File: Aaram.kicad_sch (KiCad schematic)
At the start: 51 parts, among them J1 Conn_01x03, J2 Conn_01x02, J3 AC_OUT, J4 SWITCH_IN, J5 5V_OUT, J6 PSU_AC_IN, J8 SPARE_PINS, K1 10A cube relay, K2 10A cube relay, K3 10A cube relay, Q1 BT136-600, Q2 2N2222A, Q3 2N2222A, Q4 2N2222A, U1 ESP32-DevKitC, U2 TLP281-4GB_F_

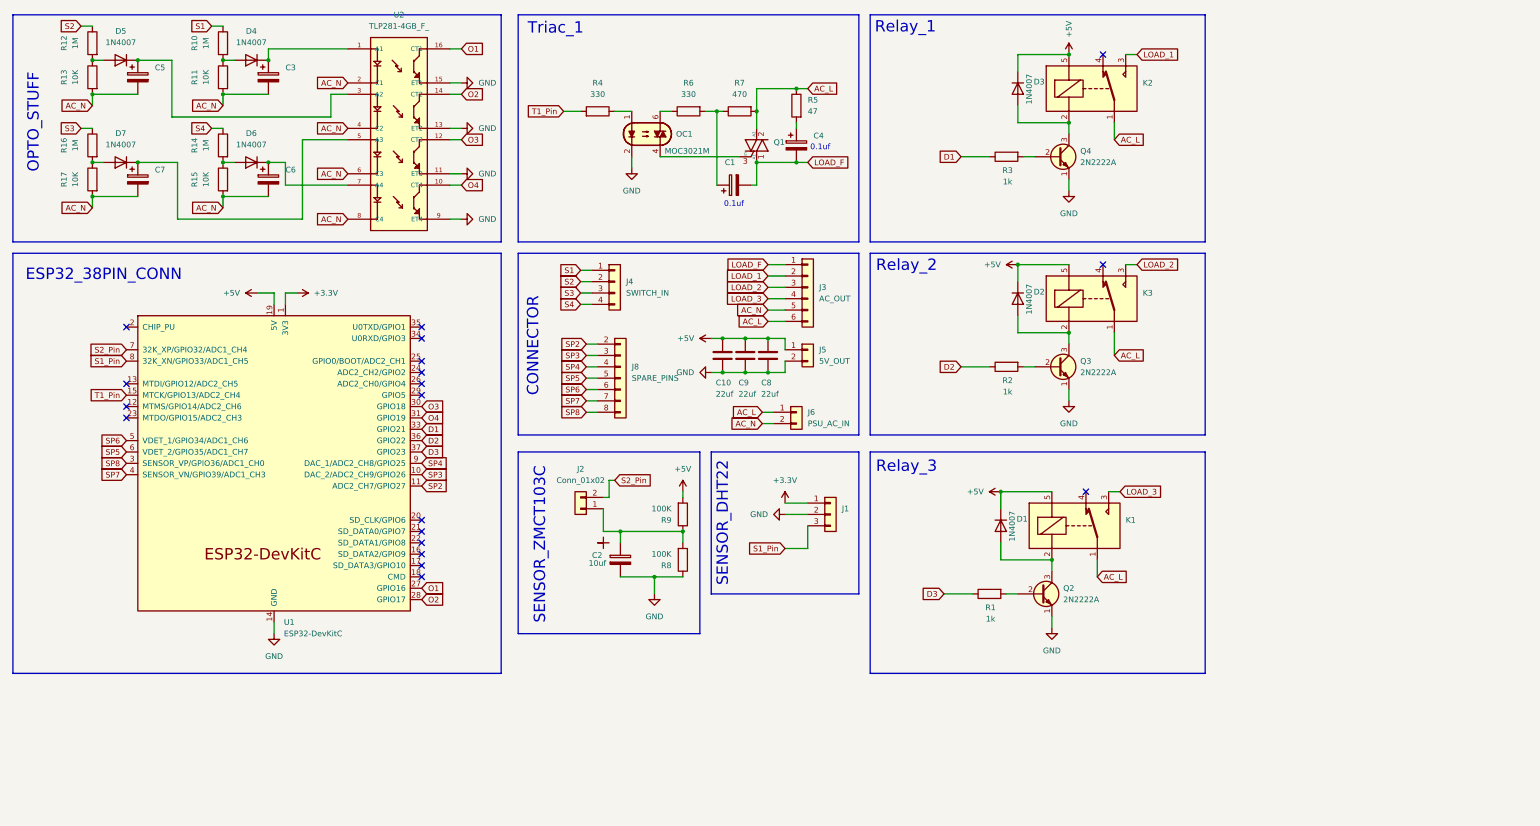
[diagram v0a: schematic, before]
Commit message: Major Update (#2)
* Updated mostly everything

* Big Update

* Major Update

- Removed All 3D related files for now.
- Updated the Schematics and PCB
- Updated the assets

* File move

* Updated readme
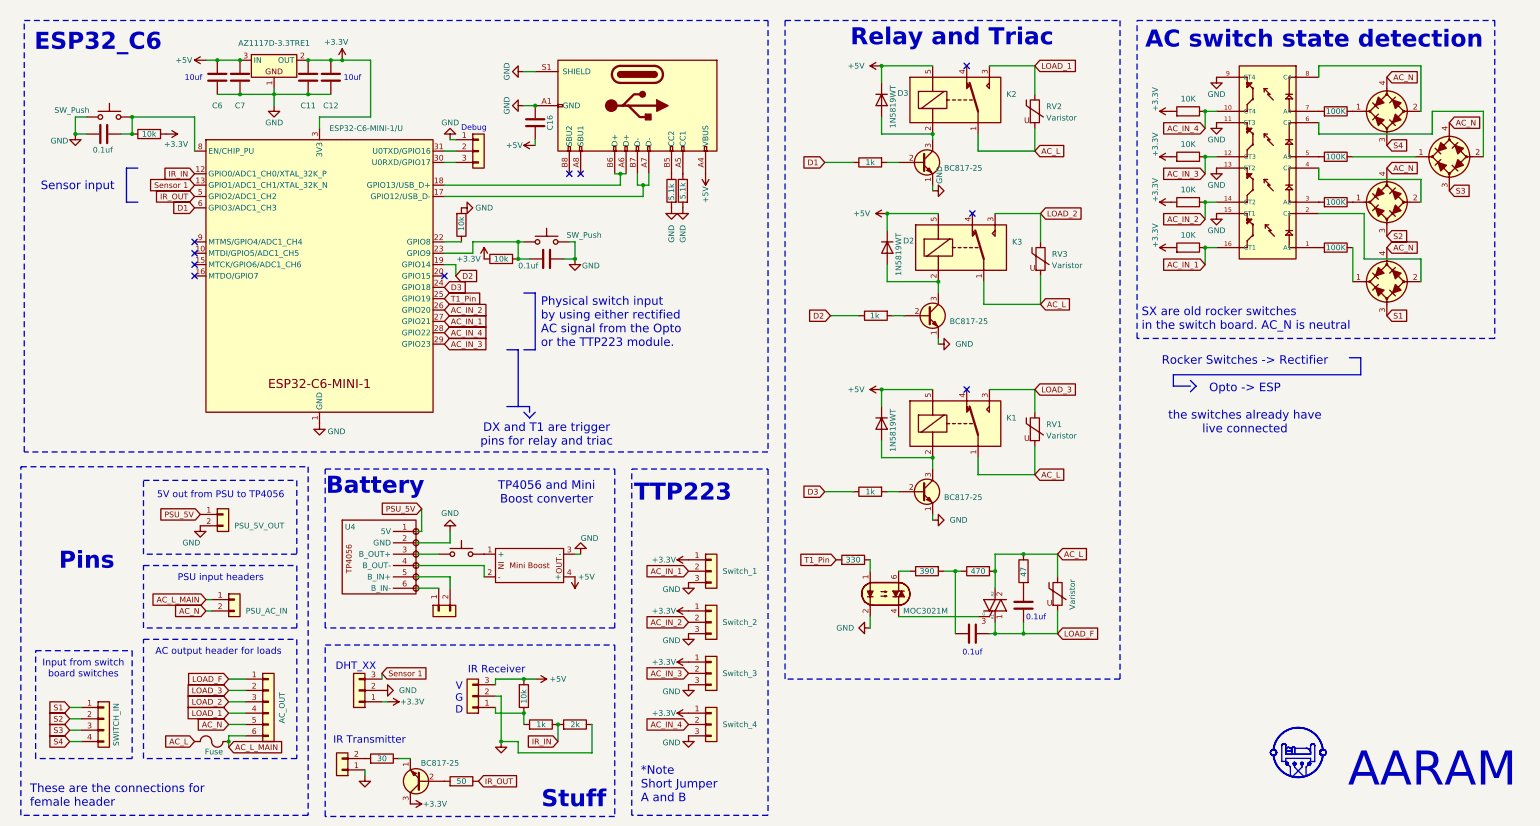
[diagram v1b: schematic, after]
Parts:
- removed C10, C8, C9: 22uf, PCM_Capacitor_SMD_Handsoldering_AKL:C_1206_3216Metric_Pad1.42x1.75mm, symbol PCM_Capacitor_AKL:C_1206
- removed C2: 10uf, Xicor_Custom stuff:Film_Cap_13x13mm_P5.00mm, symbol PCM_Capacitor_AKL:CP_Radial_D10.0mm_P5.00mm
- removed C3, C5, C6, C7: CP_Axial_L10.0mm_D4.5mm_P15.00mm, Xicor_Custom stuff:Axial_Capacitor_P10mm_W4.5mm, symbol PCM_Capacitor_AKL:CP_Axial_L10.0mm_D4.5mm_P15.00mm
- removed D4, D5, D6, D7: 1N4007, Diode_SMD:D_SMA_Handsoldering, symbol Diode:1N4007
- removed J8: SPARE_PINS, Connector_PinHeader_2.54mm:PinHeader_1x08_P2.54mm_Vertical, symbol Connector_Generic:Conn_01x08
- removed U1: ESP32-DevKitC, Xicor_Custom stuff:ESP32_38Pin, symbol PCM_Espressif:ESP32-DevKitC
- removed U2: TLP281-4GB_F_, Xicor_Custom stuff:SOIC127P700X210-16N, symbol TLP281-4GB_F_:TLP281-4GB_F_
- added C11, C12, C6, C7: 10uf, PCM_Capacitor_SMD_Handsoldering_AKL:C_1206_3216Metric_Pad1.42x1.75mm, symbol PCM_Capacitor_AKL:C_Generic
- added C16: 1uf, PCM_Capacitor_SMD_Handsoldering_AKL:C_1206_3216Metric_Pad1.42x1.75mm, symbol PCM_Capacitor_AKL:C_Generic
- added C18, C19: 0.1uf, PCM_Capacitor_SMD_Handsoldering_AKL:C_1206_3216Metric_Pad1.42x1.75mm, symbol PCM_Capacitor_AKL:C_1206
- added D10, D11, D8, D9: MB6S, PCM_Diode_SMD_AKL:Diode_Bridge_MBS, symbol PCM_Diode_Bridge_AKL:MB6S
- added F1: Fuse, Xicor_Custom stuff:BLX-A, symbol PCM_Device_AKL:Fuse
- added J10, J11: Conn_01x03, Connector_PinSocket_2.54mm:PinSocket_1x03_P2.54mm_Vertical, symbol Connector_Generic:Conn_01x03
- added J8: USB_C_Receptacle_USB2.0_16P, Connector_USB:USB_C_Receptacle_GCT_USB4105-xx-A_16P_TopMnt_Horizontal, symbol Connector:USB_C_Receptacle_USB2.0_16P
- added J9: Conn_01x02, Connector_PinSocket_2.54mm:PinSocket_1x02_P2.54mm_Vertical, symbol Connector_Generic:Conn_01x02
- added Q5: BC817-25, Package_TO_SOT_SMD:TSOT-23_HandSoldering, symbol PCM_Transistor_BJT_AKL:2N2222A
- added R19, R23: 100K, PCM_Resistor_SMD_AKL:R_2512_6332Metric_Pad1.52x3.35mm_HandSolder, symbol PCM_Resistor_AKL:R_1206
- added R20, R25, R26, R27: 10K, PCM_Resistor_SMD_AKL:R_1206_3216Metric_Pad1.42x1.75mm_HandSolder, symbol PCM_Resistor_AKL:R_1206
- added R21, R22: 10k, PCM_Resistor_SMD_AKL:R_1206_3216Metric_Pad1.42x1.75mm_HandSolder, symbol PCM_Resistor_AKL:R_1206
- added RV1, RV2, RV3, RV4: Varistor, Xicor_Custom stuff:Varistor_10D431K, symbol Device:Varistor
- added SW1, SW4: SW_Push, Xicor_Custom stuff:Tactile switch 6x3, symbol Switch:SW_Push
- added SW2: SW_Push, Xicor_Custom stuff:SMD Tactile switch, symbol Switch:SW_Push
- added Switch_1, Switch_2, Switch_3, Switch_4: Conn_01x03_Socket, Connector_JST:JST_SH_BM03B-SRSS-TB_1x03-1MP_P1.00mm_Vertical, symbol Connector_Generic:Conn_01x03
- added U1: ESP32-C6-MINI-1/U, PCM_Espressif:ESP32-C6-MINI-1, symbol PCM_Espressif:ESP32-C6-MINI-1/U
- added U2: AZ1117D-3.3TRE1, PCM_Package_TO_SOT_SMD_AKL:TO-252-2, symbol PCM_Voltage_Regulator_AKL:AZ1117D-3.3TRE1
- added U3: ~, Xicor_Custom stuff:Mini_Boost, symbol Xicor_Custom:Mini_Boost
- added U4: ~, Xicor_Custom stuff:TP4056-18650, symbol Xicor_Custom:TP4056-18650
- added U5: TLP281-4GB_F_, Xicor_Custom stuff:SOP127P780X200-16N, symbol TLP281-4GB_F_:TLP281-4GB_F_
- C1: symbol PCM_Capacitor_AKL:CP_Axial_L10.0mm_D4.5mm_P15.00mm -> PCM_Capacitor_AKL:C_3640
- C4: symbol PCM_Capacitor_AKL:CP_Axial_L10.0mm_D4.5mm_P15.00mm -> PCM_Capacitor_US_AKL:C_0805
- D1, D2, D3: value 1N4007 -> 1N5819WT
- J5: value 5V_OUT -> PSU_5V_OUT
- Q2, Q3, Q4: value 2N2222A -> BC817-25; footprint PCM_Package_TO_SOT_SMD_AKL:SOT-23_BigPads -> Package_TO_SOT_SMD:TSOT-23_HandSoldering
- R1, R2, R3, R4: footprint PCM_Capacitor_SMD_Handsoldering_AKL:C_1206_3216Metric_Pad1.42x1.75mm -> PCM_Resistor_SMD_AKL:R_1206_3216Metric_Pad1.42x1.75mm_HandSolder
- R10, R16: value 1M -> 10k; footprint PCM_Capacitor_SMD_Handsoldering_AKL:C_1206_3216Metric_Pad1.42x1.75mm -> PCM_Resistor_SMD_AKL:R_1206_3216Metric_Pad1.42x1.75mm_HandSolder
- R11: value 10K -> 30; footprint PCM_Capacitor_SMD_Handsoldering_AKL:C_1206_3216Metric_Pad1.42x1.75mm -> PCM_Resistor_SMD_AKL:R_1206_3216Metric_Pad1.42x1.75mm_HandSolder
- R12, R14: value 1M -> 5.1k; footprint PCM_Capacitor_SMD_Handsoldering_AKL:C_1206_3216Metric_Pad1.42x1.75mm -> PCM_Resistor_SMD_AKL:R_1206_3216Metric_Pad1.42x1.75mm_HandSolder
- R13: value 10K -> 50; footprint PCM_Capacitor_SMD_Handsoldering_AKL:C_1206_3216Metric_Pad1.42x1.75mm -> PCM_Resistor_SMD_AKL:R_1206_3216Metric_Pad1.42x1.75mm_HandSolder
- R15, R17: value 10K -> 100K; footprint PCM_Capacitor_SMD_Handsoldering_AKL:C_1206_3216Metric_Pad1.42x1.75mm -> PCM_Resistor_SMD_AKL:R_2512_6332Metric_Pad1.52x3.35mm_HandSolder
- R5, R7: footprint PCM_Capacitor_SMD_Handsoldering_AKL:C_1206_3216Metric_Pad1.42x1.75mm -> PCM_Resistor_SMD_AKL:R_2512_6332Metric_Pad1.52x3.35mm_HandSolder
- R6: value 330 -> 390; footprint PCM_Capacitor_SMD_Handsoldering_AKL:C_1206_3216Metric_Pad1.42x1.75mm -> PCM_Resistor_SMD_AKL:R_2512_6332Metric_Pad1.52x3.35mm_HandSolder
- R8: value 100K -> 2k; footprint PCM_Capacitor_SMD_Handsoldering_AKL:C_1206_3216Metric_Pad1.42x1.75mm -> PCM_Resistor_SMD_AKL:R_1206_3216Metric_Pad1.42x1.75mm_HandSolder
- R9: value 100K -> 1k; footprint PCM_Capacitor_SMD_Handsoldering_AKL:C_1206_3216Metric_Pad1.42x1.75mm -> PCM_Resistor_SMD_AKL:R_1206_3216Metric_Pad1.42x1.75mm_HandSolder
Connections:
- net +3.3V: now also R10.1, C11.2, C12.2, Q5.3 (C), R20.1, R21.2, R25.1, R26.1, R27.1, Switch_1.1 (Pin_1), Switch_2.1 (Pin_1), Switch_3.1 (Pin_1), Switch_4.1 (Pin_1), U1.3 (3V3), U2.2 (OUT)
- net +5V: now also R16.1, C16.1, C6.2, C7.2, J10.3 (Pin_3), J8.A4 (VBUS), J8.A9 (VBUS), J8.B4 (VBUS), J8.B9 (VBUS), U2.3 (IN), U3.4 (+); no longer J5.1 (Pin_1), R9.1
- net AC_L: now also F1.1, RV1.2, RV2.2, RV3.2, RV4.1; no longer J3.6 (Pin_6), J6.1 (Pin_1)
- net AC_N: now also D10.4 (2), D11.4 (2), D8.4 (2), D9.4 (2); no longer R11.1, R13.1, R15.1, R17.1
- net D1: now also R2.2, U1.6 (GPIO3/ADC1_CH3); no longer R3.2
- net D2: now also R1.2, U1.19 (GPIO14); no longer R2.2
- net D3: now also R3.2, U1.24 (GPIO18); no longer R1.2
- net GND: now also J2.1 (Pin_1), R12.1, R14.1, C11.1, C12.1, C16.2, C18.1, C19.1, C6.1, C7.1, J10.2 (Pin_2), J11.1 (Pin_1), J8.A1 (GND), J8.A12 (GND), J8.B1 (GND), J8.B12 (GND), J8.S1 (SHIELD), R22.1, SW1.1, SW4.1, Switch_1.3 (Pin_3), Switch_2.3 (Pin_3), Switch_3.3 (Pin_3), Switch_4.3 (Pin_3), U1.1 (GND), U1.11 (GND), U1.14 (GND), U1.2 (GND), U1.36 (GND), U1.37 (GND), U1.38 (GND), U1.39 (GND), U1.40 (GND), U1.41 (GND), U1.42 (GND), U1.43 (GND), U1.44 (GND), U1.45 (GND), U1.46 (GND), U1.47 (GND), U1.48 (GND), U1.49 (GND), U1.50 (GND), U1.51 (GND), U1.52 (GND), U1.53 (GND), U2.1, U3.3 (-), U4.2 (GND), U5.11 (ET3), U5.13 (ET2), U5.15 (ET1), U5.9 (ET4)
- net LOAD_1: now also J3.4 (Pin_4), RV2.1; no longer J3.2 (Pin_2)
- net LOAD_2: now also RV3.1
- net LOAD_3: now also J3.2 (Pin_2), RV1.1; no longer J3.4 (Pin_4)
- net LOAD_F: now also RV4.2
- net S1: now also D8.3 (1); no longer R10.2
- net S2: now also D9.3 (1); no longer R12.2
- net S3: now also D10.3 (1); no longer R16.2
- net S4: now also D11.3 (1); no longer R14.2
- net T1_Pin: now also U1.25 (GPIO19)
- net at D2.2 (A), K3.2: now also Q2.3 (C); no longer Q3.3 (C)
- net at R11.2: now also Q5.1 (E); no longer R10.1
- net at R15.2: now also D9.1 (+); no longer R14.1
- net at R17.2: now also D10.1 (+); no longer R16.1
- net IR_OUT: now reaches R13.2
- net IR_OUT: now also U1.5 (GPIO2/ADC1_CH2); no longer R12.1
- net at D3.2 (A), K2.2: now also Q3.3 (C); no longer Q4.3 (C)
- net IR_IN: now reaches R8.1, R9.2
- net IR_IN: now also U1.12 (GPIO0/ADC1_CH0/XTAL_32K_P); no longer J2.1 (Pin_1)
- net at D1.2 (A), K1.2: now also Q4.3 (C); no longer Q2.3 (C)
- net S1_Pin renamed Sensor 1
- net Sensor 1: now also U1.13 (GPIO1/ADC1_CH1/XTAL_32K_N)
- net S2_Pin: no longer names the net of J2.2 (Pin_2)
- net S2_Pin: now also R11.1
- new net: J8.A5 (CC1), R12.2
- new net: J8.A6 (D+), J8.B6 (D+), U1.18 (GPIO13/USB_D+)
- new net: J8.A7 (D-), J8.B7 (D-), U1.17 (GPIO12/USB_D-)
- new net: J8.B5 (CC2), R14.2
- new net: R19.1, U5.7 (A4)
- new net: D11.1 (+), R19.2
- new net: Q5.2 (B), R13.1
- new net: C19.2, R21.1, SW4.2, U1.23 (GPIO9)
- new net: C18.2, R10.2, SW1.2, U1.8 (EN/CHIP_PU)
- new net: SW2.1, U3.1 (+)
- new net: U3.2 (-), U4.4 (B_OUT-)
- new net: D8.1 (+), R23.2
- new net: D8.2 (-), U5.2 (C1)
- new net: R15.1, U5.3 (A2)
- new net: R23.1, U5.1 (A1)
- new net: D9.2 (-), U5.4 (C2)
- new net: R17.1, U5.5 (A3)
- new net: D10.2 (-), U5.6 (C3)
- new net: D11.2 (-), U5.8 (C4)
- new net: J9.1 (Pin_1), U4.6 (B_IN-)
- new net: J9.2 (Pin_2), U4.5 (B_IN+)
- new net: R22.2, U1.22 (GPIO8)
- new net: J10.1 (Pin_1), R16.2, R9.1
- new net: J11.2 (Pin_2), U1.31 (U0TXD/GPIO16)
- new net: J11.3 (Pin_3), U1.30 (U0RXD/GPIO17)
- new net: SW2.2, U4.3 (B_OUT+)
- new net AC_IN_1: R26.2, Switch_1.2 (Pin_2), U1.27 (GPIO21), U5.16 (CT1)
- new net AC_IN_2: R25.2, Switch_2.2 (Pin_2), U1.26 (GPIO20), U5.14 (CT2)
- new net AC_IN_3: R20.2, Switch_3.2 (Pin_2), U1.29 (GPIO23), U5.12 (CT3)
- new net AC_IN_4: R27.2, Switch_4.2 (Pin_2), U1.28 (GPIO22), U5.10 (CT4)
- new net AC_L_MAIN: F1.2, J3.6 (Pin_6), J6.1 (Pin_1)
- new net PSU_5V: J5.1 (Pin_1), U4.1 (5V)
- no-connect marks 19 -> 10
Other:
- note added: "*Note Short Jumper A and B"
- note added: "10uf"
- note added: "5V out from PSU to TP4056"
- note added: "AARAM"
- note added: "AC output header for loads"
- note added: "AC switch state detection"
- note added: "Battery"
- note added: "DHT_XX"
- note added: "DX and T1 are trigger pins for relay and triac"
- note added: "Debug"
- note added: "ESP32_C6"
- note added: "IR Receiver"
- note added: "IR Transmitter"
- note added: "Input from switch board switches"
- note added: "PSU input headers"
- note added: "Physical switch input by using either rectified AC signal from the Opto or the TTP223 module."
- note added: "Pins"
- note added: "Relay and Triac"
- note added: "Rocker Switches -> Rectifier Opto -> ESP the switches already have live connected"
- note added: "SX are old rocker switches in the switch board. AC_N is neutral"
- note added: "Sensor input"
- note added: "Stuff"
- note added: "TP4056 and Mini Boost converter"
- note added: "TTP223"
- note added: "These are the connections for female header"
- note added: "V G D"
- note removed: "CONNECTOR"
- note removed: "ESP32_38PIN_CONN"
- note removed: "OPTO_STUFF"
- note removed: "Relay_1"
- note removed: "Relay_2"
- note removed: "Relay_3"
- note removed: "SENSOR_DHT22"
- note removed: "SENSOR_ZMCT103C"
- note removed: "Triac_1"
- title: (none) -> Aaram - Home Automation
- moved on the sheet: D2, D3, K1, K2, K3
